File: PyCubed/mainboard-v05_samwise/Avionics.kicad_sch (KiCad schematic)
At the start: 27 parts, among them SW1 KMR231NG LFS, U1 MAX706RESA, U2 ATSAMD51J20A-AU, Y1 32.768kHz

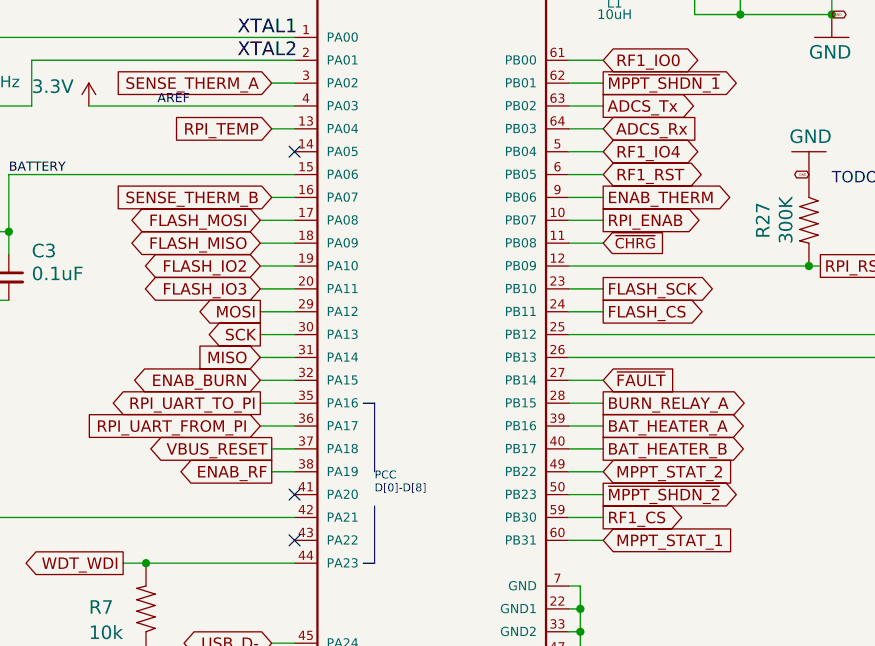
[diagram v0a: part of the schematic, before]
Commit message: Layout and Routing work
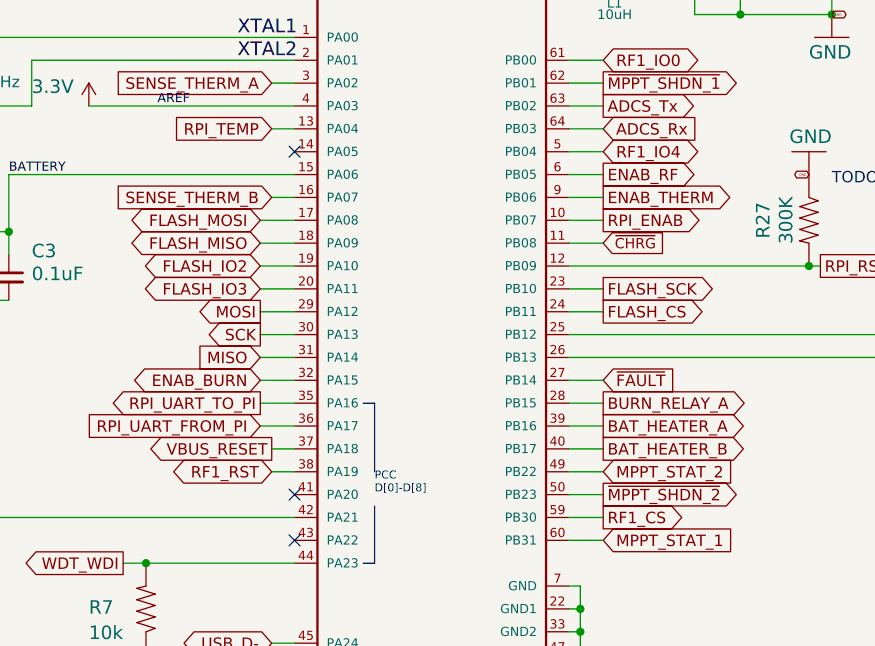
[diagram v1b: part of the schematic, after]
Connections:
- net ENAB_RF: now also U2.6 (PB05); no longer U2.38 (PA19)
- net RF1_RST: now also U2.38 (PA19); no longer U2.6 (PB05)
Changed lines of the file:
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@@
+    (stroke (width 0) (type default))
+  )
+  (wire (pts (xy 123.19 120.65) (xy 127 120.65))
     (stroke (width 0) (type default))
   )
@@
     (stroke (width 0) (type default))
   )
+  (wire (pts (xy 90.17 153.67) (xy 92.71 153.67))
+    (stroke (width 0) (type default))
+  )
   (wire (pts (xy 27.94 166.37) (xy 41.91 166.37))
     (stroke (width 0) (type default))
@@
     (stroke (width 0) (type default))
   )
-  (wire (pts (xy 127 120.65) (xy 123.19 120.65))
-    (stroke (width 0) (type default))
-  )
   (wire (pts (xy 49.53 113.03) (xy 63.5 113.03))
     (stroke (width 0) (type default))
@@
   )
   (wire (pts (xy 123.19 173.99) (xy 124.46 173.99))
-    (stroke (width 0) (type default))
-  )
-  (wire (pts (xy 92.71 153.67) (xy 90.17 153.67))
     (stroke (width 0) (type default))
   )
@@
     )
   )
-  (global_label "ENAB_RF" (shape output) (at 90.17 153.67 180) (fields_autoplaced)
-    (effects (font (size 1.27 1.27)) (justify right))
-    (property "Intersheetrefs" "${INTERSHEET_REFS}" (at 79.6747 153.67 0)
-      (effects (font (size 1.27 1.27)) (justify right) hide)
+  (global_label "ENAB_RF" (shape output) (at 127 120.65 0) (fields_autoplaced)
+    (effects (font (size 1.27 1.27)) (justify left))
+    (property "Intersheetrefs" "${INTERSHEET_REFS}" (at 137.4953 120.65 0)
+      (effects (font (size 1.27 1.27)) (justify left) hide)
     )
   )
@@
     )
   )
-  (global_label "RF1_RST" (shape bidirectional) (at 127 120.65 0) (fields_autoplaced)
-    (effects (font (size 1.27 1.27)) (justify left))
-    (property "Intersheetrefs" "${INTERSHEET_REFS}" (at 137.3071 120.5706 0)
-      (effects (font (size 1.27 1.27)) (justify left) hide)
-    )
-  )
+  (global_label "RF1_RST" (shape bidirectional) (at 90.17 153.67 180) (fields_autoplaced)
+    (effects (font (size 1.27 1.27)) (justify right))
+    (property "Intersheetrefs" "${INTERSHEET_REFS}" (at 78.9037 153.67 0)
+      (effects (font (size 1.27 1.27)) (justify right) hide)
+    )
+  )
